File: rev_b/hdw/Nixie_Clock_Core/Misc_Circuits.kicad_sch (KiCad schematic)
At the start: 20 parts, among them U2401 LTC6900, U2402 74LVC1G08

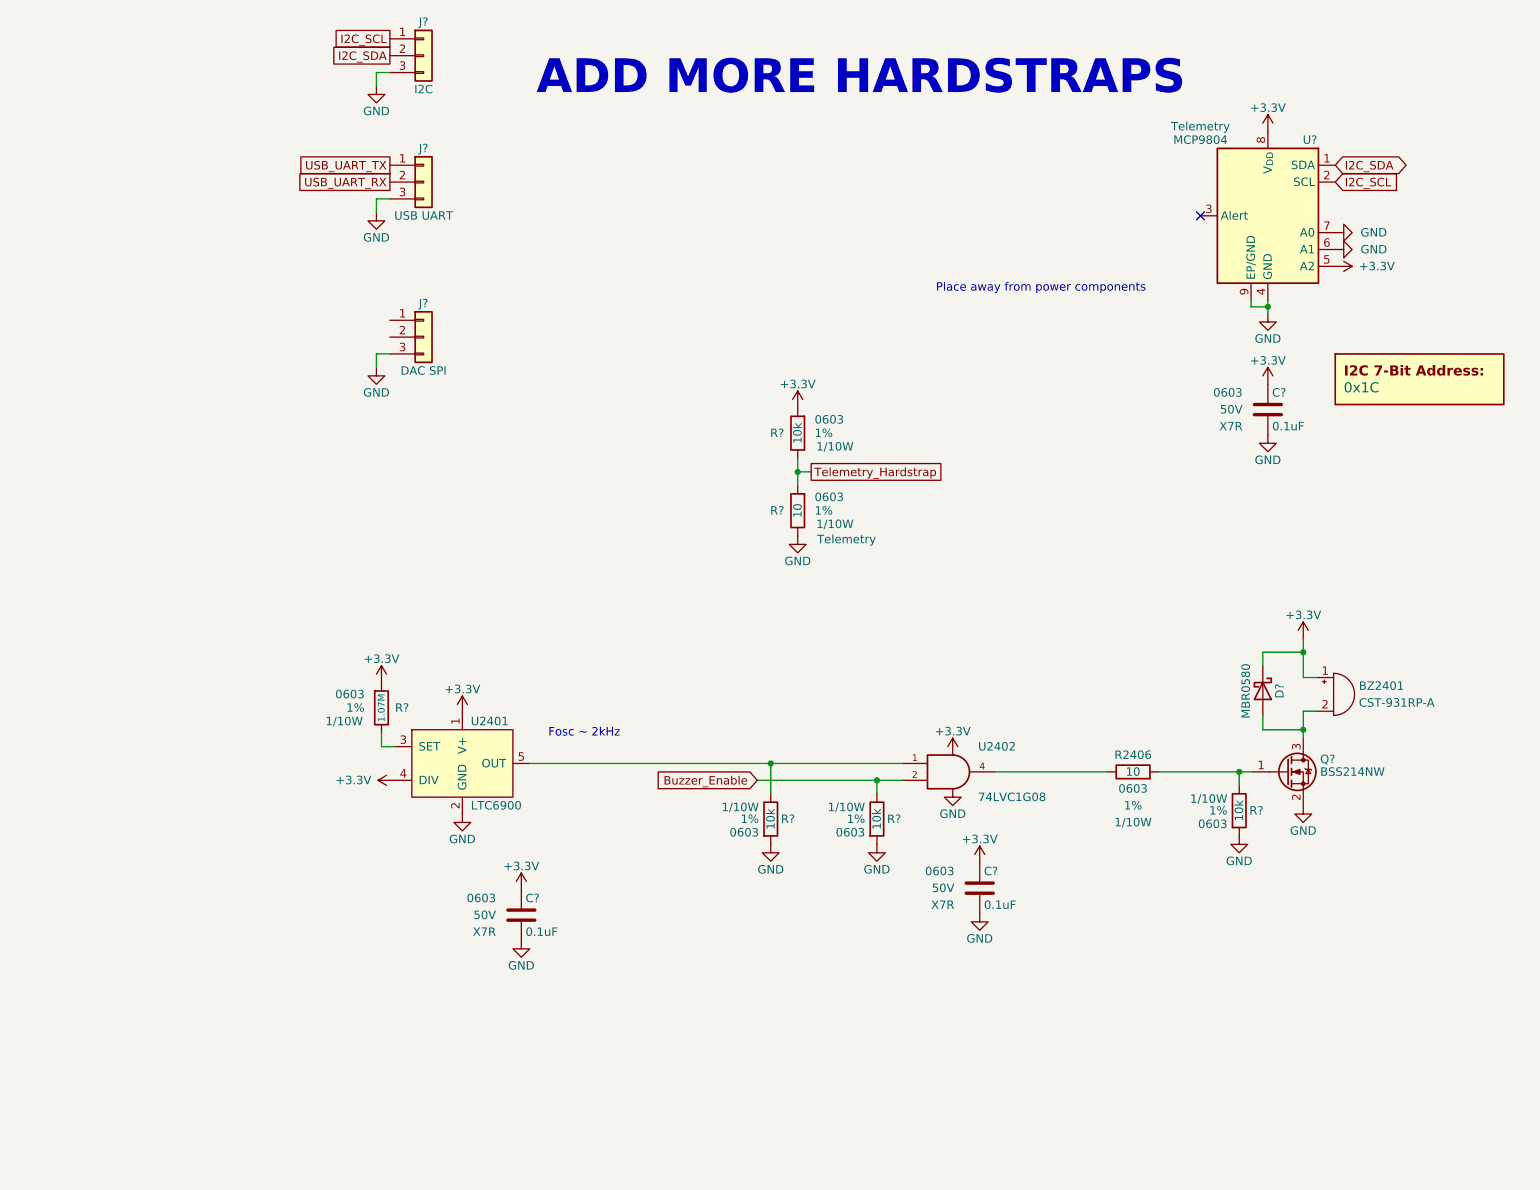
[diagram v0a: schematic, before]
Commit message: lots of rev B control board schematic progress
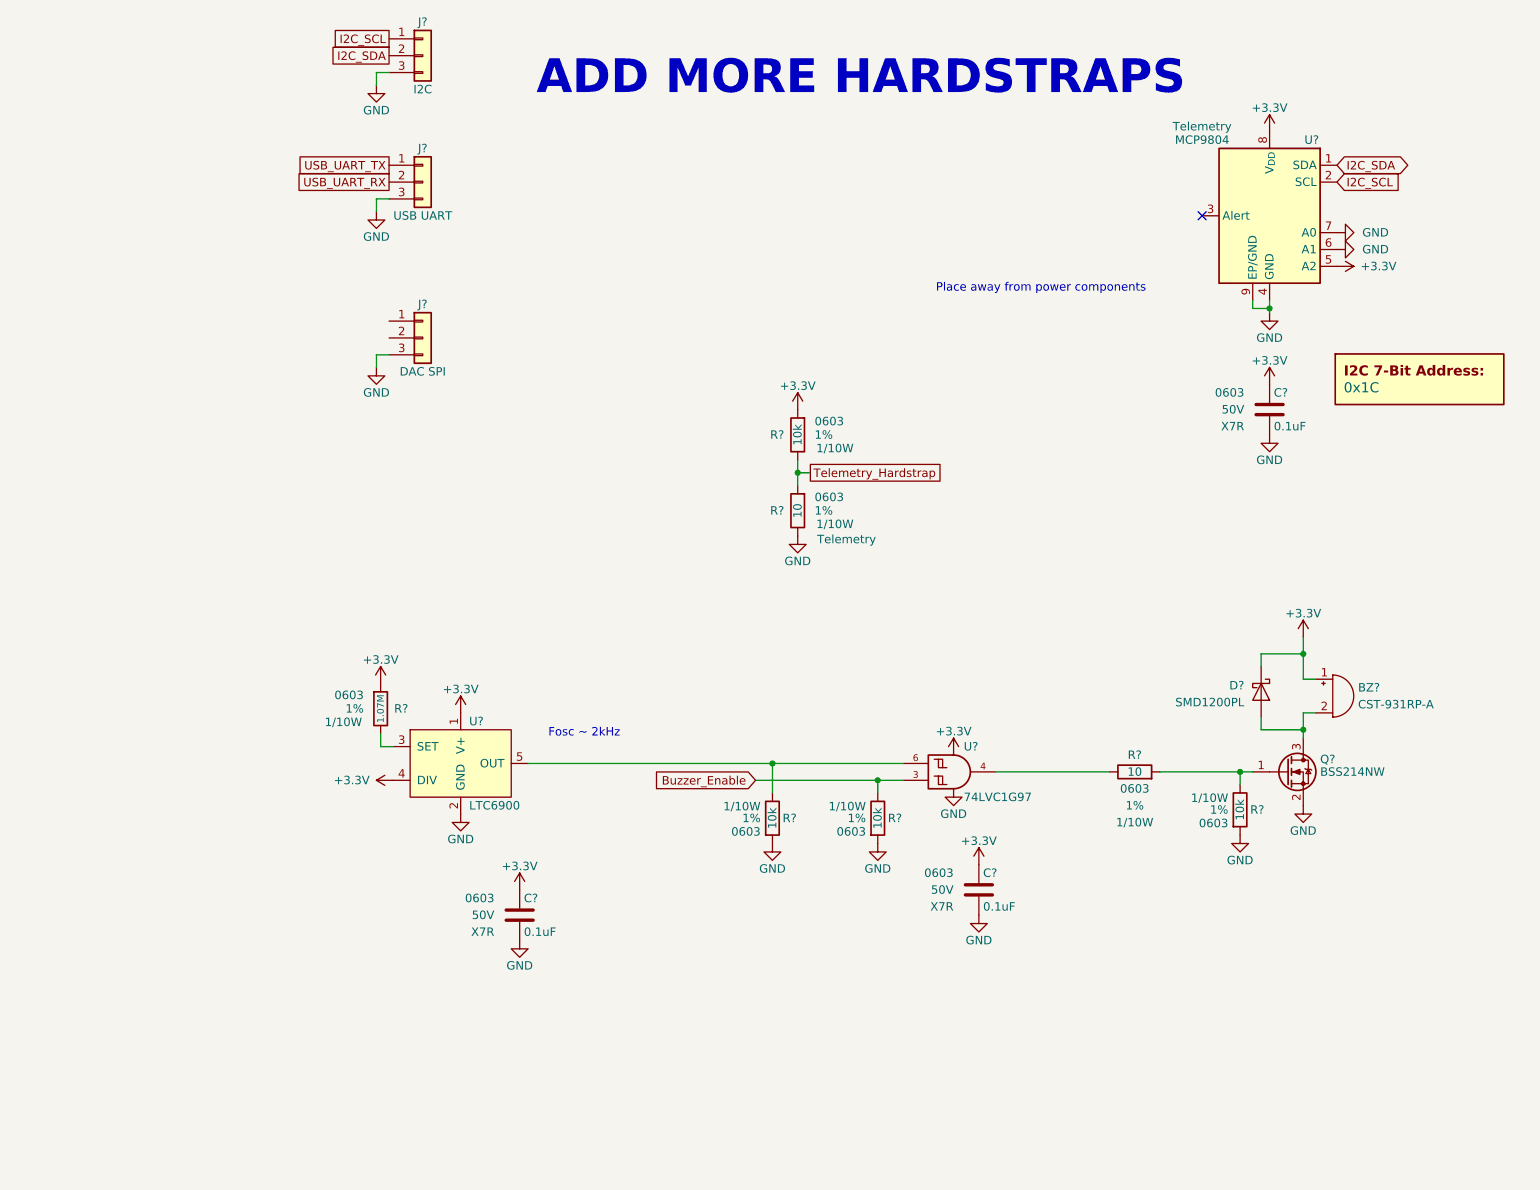
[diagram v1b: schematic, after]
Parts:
- removed D?: MBR0580, Diode_SMD:D_SOD-123, symbol Diode:MBR0580
- removed U2402: 74LVC1G08, Package_TO_SOT_SMD:SOT-353_SC-70-5, symbol Custom_Library:74LVC1G08_Power
- added D?: SMD1200PL, Diodes_SMD:D_SOD-123F, symbol Nixie-Clock-rescue:D_Schottky
- added U?: 74LVC1G97, Package_TO_SOT_SMD:SOT-363_SC-70-6, symbol Custom Library:74LVC1G97_Power_AND
- renumbered BZ2401 to BZ?, R2406 to R?, U2401 to U?
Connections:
- net +3.3V: now also D?.1 (K), U?.5 (VCC)
- net Buzzer_Enable: now also U?.3
- net GND: now also U?.1 (GND), U?.2 (GND)
- net at BZ?.2 (+), Q?.3 (D): now also D?.2 (A)
- net at R?.2, U?.5 (OUT): now also U?.6
- net at R?.2: now also U?.4

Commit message: more rev b sch progress
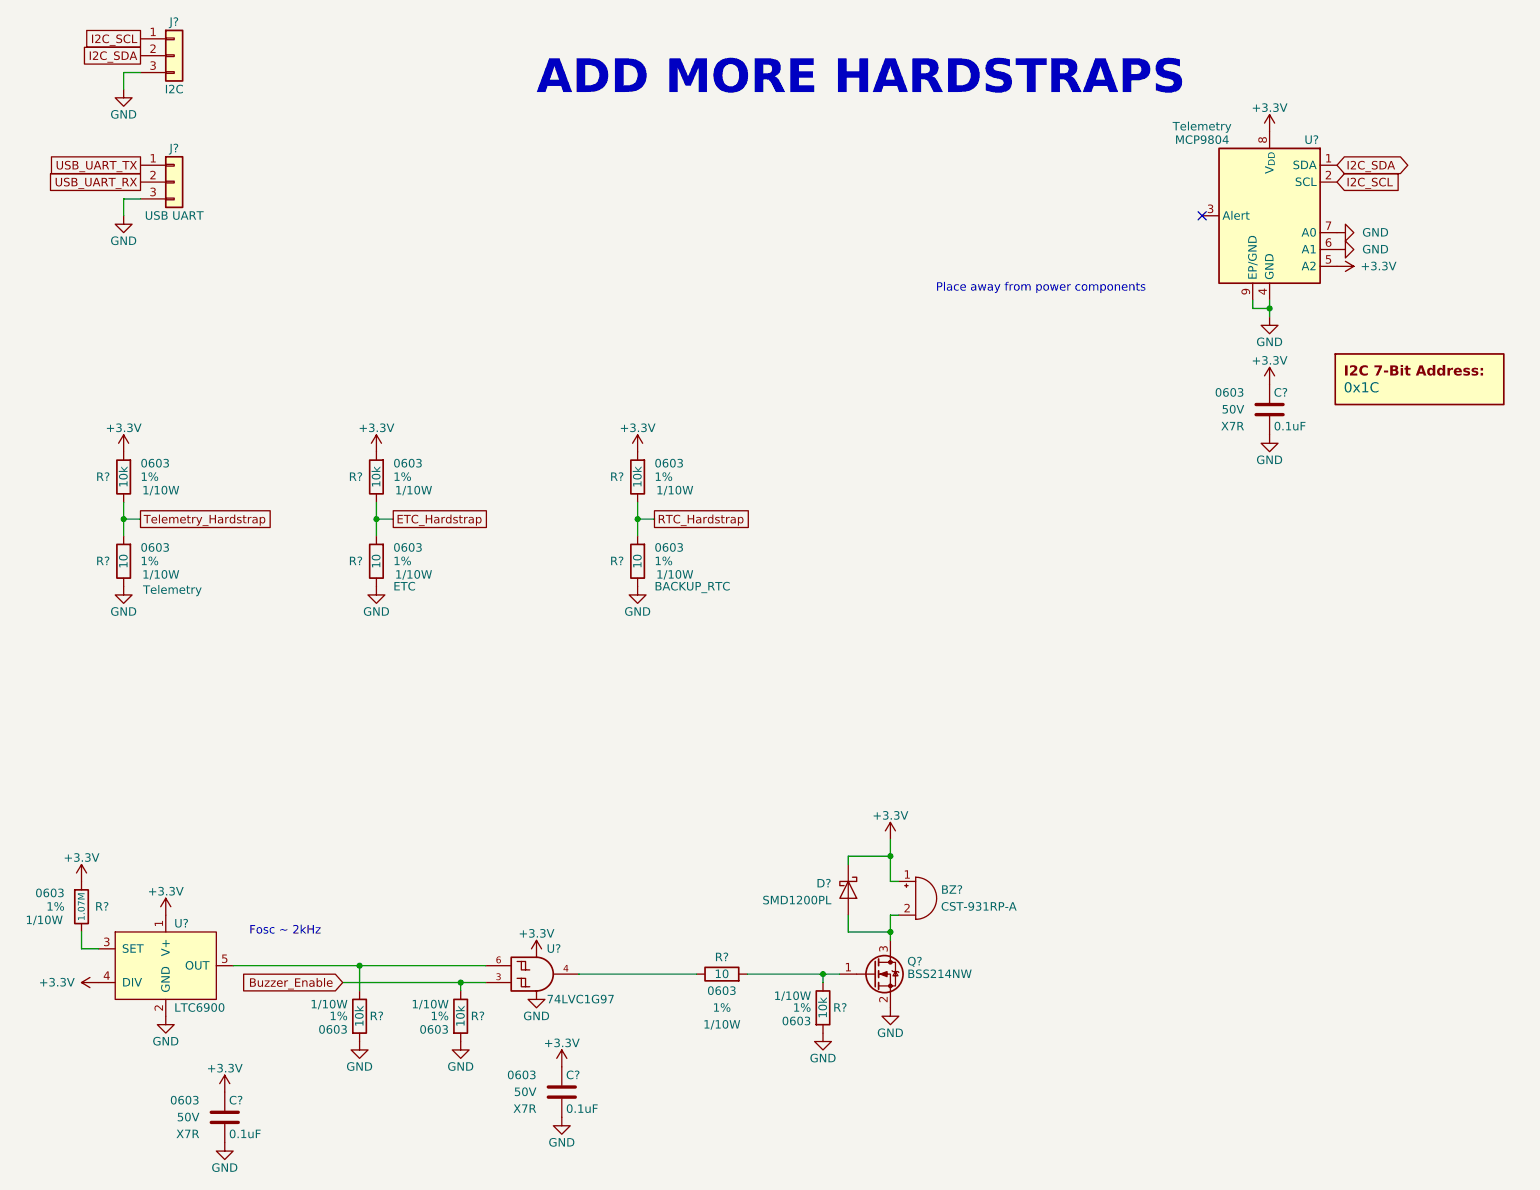
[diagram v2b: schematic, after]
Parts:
- removed J?: DAC SPI, Pin_Headers:Pin_Header_Straight_1x03_Pitch2.54mm, symbol Connector_Generic:Conn_01x03
- added R? (x2): 10k, Resistors_SMD:R_0603, symbol Custom_Library:R_Custom
- added R? (x2): 10, Resistors_SMD:R_0603, symbol Custom_Library:R_Custom
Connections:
- net +3.3V: now also R?.1, R?.1
- net GND: now also R?.2, R?.2
- new net ETC_Hardstrap: R?.1, R?.2
- new net RTC_Hardstrap: R?.1, R?.2
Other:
- moved on the sheet: BZ?, C?, D?, J?, Q?, R?, U?
